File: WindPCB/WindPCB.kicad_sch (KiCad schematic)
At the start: 24 parts, among them J1 1267, J2 1267, J3 1267, J4 1267, J5 1267, J6 Conn_01x04, U1 LM7808_TO220, U3 LM7805_TO220, U4 MCP2562-E-P, U5 ESP32-C3_SUPERMINI

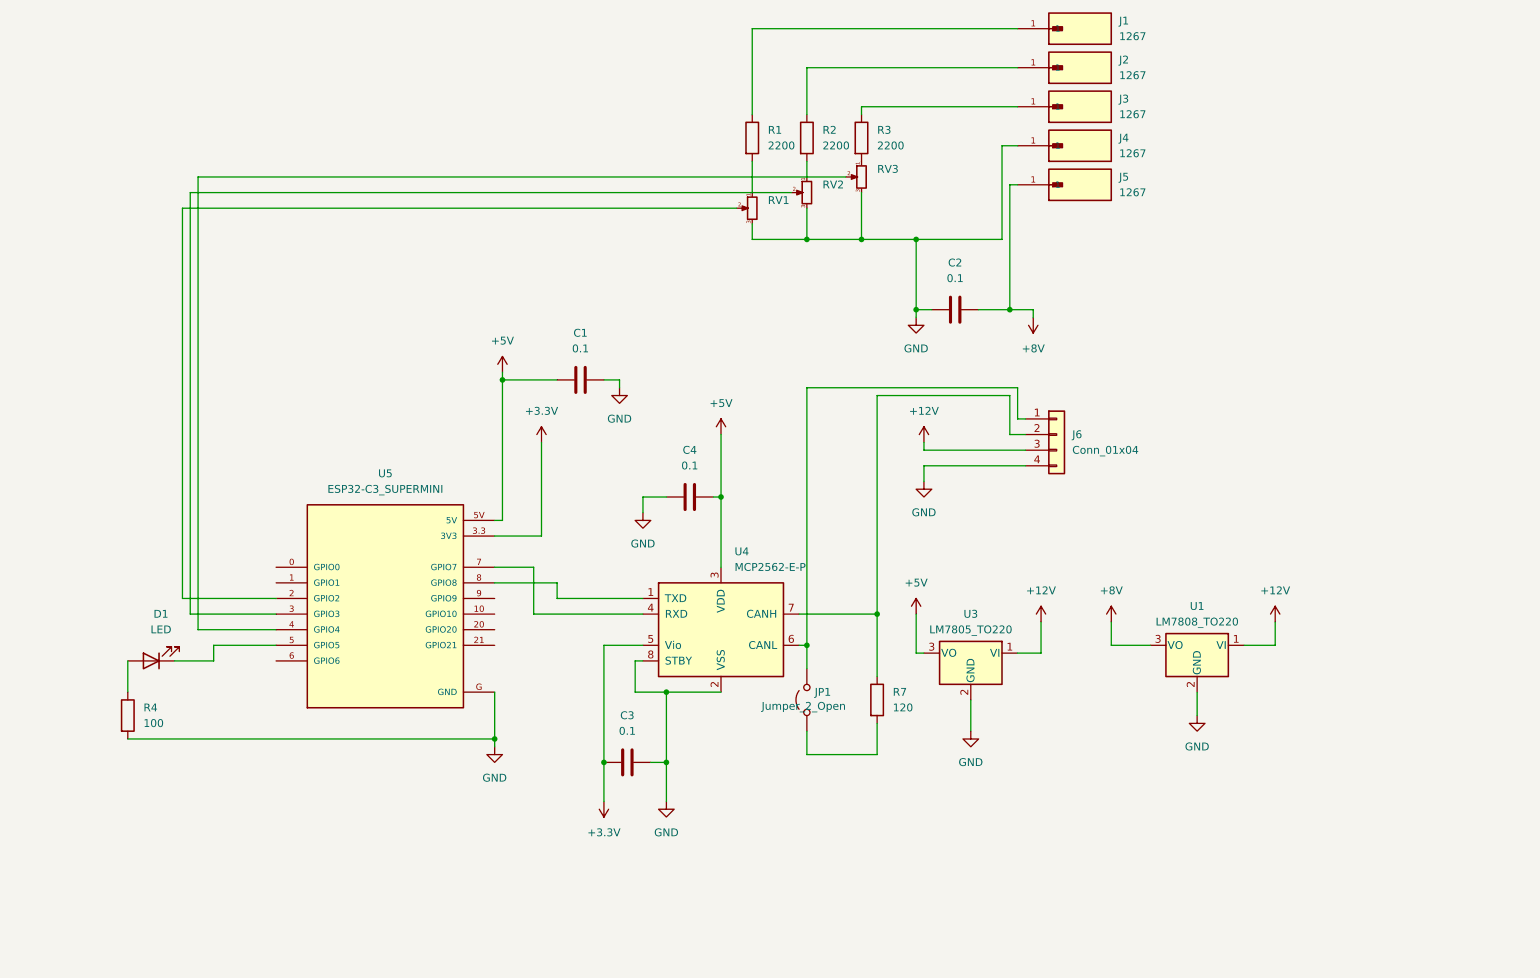
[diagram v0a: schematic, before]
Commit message: Lot of good stuff
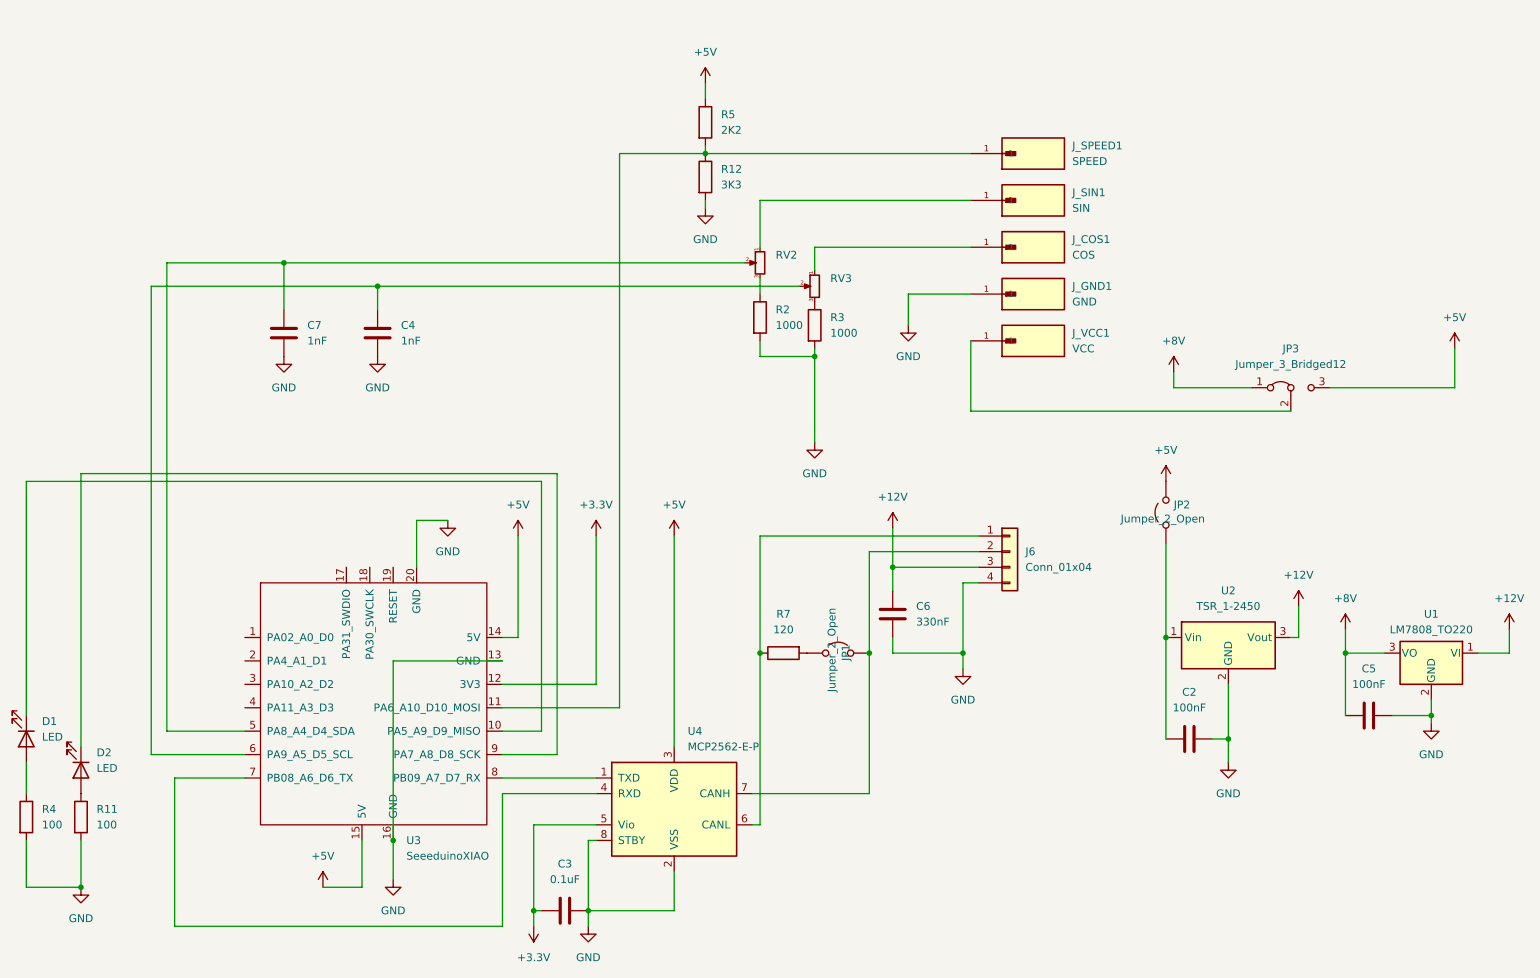
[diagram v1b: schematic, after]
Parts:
- removed C1: 0.1, Capacitor_THT:C_Disc_D6.0mm_W2.5mm_P5.00mm, symbol Device:C
- removed R1: 2200, Resistor_THT:R_Axial_DIN0204_L3.6mm_D1.6mm_P7.62mm_Horizontal, symbol Device:R
- removed RV1: R_Potentiometer_Small, Potentiometer_THT:Potentiometer_Bourns_3296W_Vertical, symbol Device:R_Potentiometer_Small
- removed U3: LM7805_TO220, Package_TO_SOT_THT:TO-220-3_Vertical, symbol Regulator_Linear:LM7805_TO220
- removed U5: ESP32-C3_SUPERMINI, Library:WAVESHARE_DEVKIT_ESP32-C3-ZERO, symbol Espressif:ESP32-C3_SUPERMINI
- added C5: 100nF, Capacitor_THT:C_Disc_D6.0mm_W2.5mm_P5.00mm, symbol Device:C
- added C6: 330nF, Capacitor_THT:C_Disc_D6.0mm_W2.5mm_P5.00mm, symbol Device:C
- added C7: 1nF, Capacitor_THT:C_Disc_D6.0mm_W2.5mm_P5.00mm, symbol Device:C
- added D2: LED, LED_THT:LED_D3.0mm, symbol Device:LED
- added JP2: Jumper_2_Open, Connector_PinHeader_2.54mm:PinHeader_1x02_P2.54mm_Vertical, symbol Jumper:Jumper_2_Open
- added JP3: Jumper_3_Bridged12, Connector_PinHeader_2.54mm:PinHeader_1x03_P2.54mm_Vertical, symbol Jumper:Jumper_3_Bridged12
- added R11: 100, Resistor_THT:R_Axial_DIN0204_L3.6mm_D1.6mm_P7.62mm_Horizontal, symbol Device:R
- added R12: 3K3, Resistor_THT:R_Axial_DIN0204_L3.6mm_D1.6mm_P7.62mm_Horizontal, symbol Device:R
- added R5: 2K2, Resistor_THT:R_Axial_DIN0204_L3.6mm_D1.6mm_P7.62mm_Horizontal, symbol Device:R
- added U2: TSR_1-2450, Converter_DCDC:Converter_DCDC_TRACO_TSR-1_THT, symbol Regulator_Switching:TSR_1-2450
- added U3: SeeeduinoXIAO, Seeeduino:Seeeduino XIAO-MOUDLE14P-2.54-21X17.8MM_1, symbol Seeduino:SeeeduinoXIAO
- C2: value 0.1 -> 100nF
- C3: value 0.1 -> 0.1uF
- C4: value 0.1 -> 1nF
- J_COS1: renamed from J3; value 1267 -> COS; footprint Library:KEYSTONE_1267 -> Custom:KEYSTONE_1267
- J_GND1: renamed from J4; value 1267 -> GND; footprint Library:KEYSTONE_1267 -> Custom:KEYSTONE_1267
- J_SIN1: renamed from J2; value 1267 -> SIN; footprint Library:KEYSTONE_1267 -> Custom:KEYSTONE_1267
- J_SPEED1: renamed from J1; value 1267 -> SPEED; footprint Library:KEYSTONE_1267 -> Custom:KEYSTONE_1267
- J_VCC1: renamed from J5; value 1267 -> VCC; footprint Library:KEYSTONE_1267 -> Custom:KEYSTONE_1267
- R2, R3: value 2200 -> 1000
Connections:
- net +12V: now also C6.1, U2.3 (Vout)
- net +3.3V: now also U3.12 (3V3)
- net +5V: now also JP2.2 (B), JP3.3 (B), R5.1, U3.14 (5V), U3.15 (5V); no longer C4.2
- net +8V: now also C5.2, JP3.1 (A); no longer C2.2, J_VCC1.1
- net GND: now also C4.2, R2.2, R3.2, C5.1, C6.2, C7.2, R11.2, R12.2, U2.2 (GND), U3.13 (GND), U3.16 (GND), U3.20 (GND); no longer C4.1, RV2.3, RV3.3
- net at J6.2 (Pin_2), U4.7 (CANH): now also JP1.2 (B); no longer R7.1
- net at D1.1 (K): now also U3.10 (PA5_A9_D9_MISO)
- net at RV2.1: now also J_SIN1.1; no longer R2.2
- net at RV2.2: now also C7.1, U3.5 (PA8_A4_D4_SDA)
- net at R2.1: now also RV2.3; no longer J_SIN1.1
- net at J6.1 (Pin_1), U4.6 (CANL): now also R7.1; no longer JP1.2 (B)
- net at J_SPEED1.1: now also R12.1, R5.2, U3.11 (PA6_A10_D10_MOSI)
- net at R3.1: now also RV3.3; no longer J_COS1.1
- net at RV3.1: now also J_COS1.1; no longer R3.2
- net at RV3.2: now also C4.1, U3.6 (PA9_A5_D5_SCL)
- net at U4.4 (RXD): now also U3.7 (PB08_A6_D6_TX)
- net at U4.1 (TXD): now also U3.8 (PB09_A7_D7_RX)
- new net: C2.2, JP2.1 (A), U2.1 (Vin)
- new net: D2.1 (K), U3.9 (PA7_A8_D8_SCK)
- new net: D2.2 (A), R11.1
- new net: JP3.2 (C), J_VCC1.1
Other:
- moved on the sheet: C2, C3, D1, J6, JP1, J_COS1, J_GND1, J_SIN1, J_SPEED1, J_VCC1, R2, R3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
